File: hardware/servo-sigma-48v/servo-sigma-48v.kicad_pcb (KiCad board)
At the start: 4 copper layers, 74.5 x 75.2 mm, 203 parts, among them J1 CONN_01X02, J10 Conn_01x03, J11 Conn_01x03, J12 Conn_01x05, J2 CONN_02X05, J3 CONN_01X03, J4 Conn_01x03, J5 Conn_01x05, J6 629_105_150_921, J7 CONN_01X02, J8 Conn_01x03, J9 Conn_01x03, Q1 STL160NS3LLH7, Q2 STL160NS3LLH7, Q3 STL160NS3LLH7, Q4 STL160NS3LLH7, Q5 STL160NS3LLH7, Q6 STL160NS3LLH7, Q7 STL160NS3LLH7, Q8 STL160NS3LLH7, SW1 SW_DIP_x04, U1 ST1S14, U10 OPA4374, U11 L6398, U12 SN65HVD75DGKR, U2 TPS70950, U3 SN65HVD75DGKR, U4 L6398, U5 STM32F405VGTx, U6 L6398, U7 L6398, U8 TPS70933, U9 OPA4374, Y1 ABM3-8.000MHZ-D2Y-T

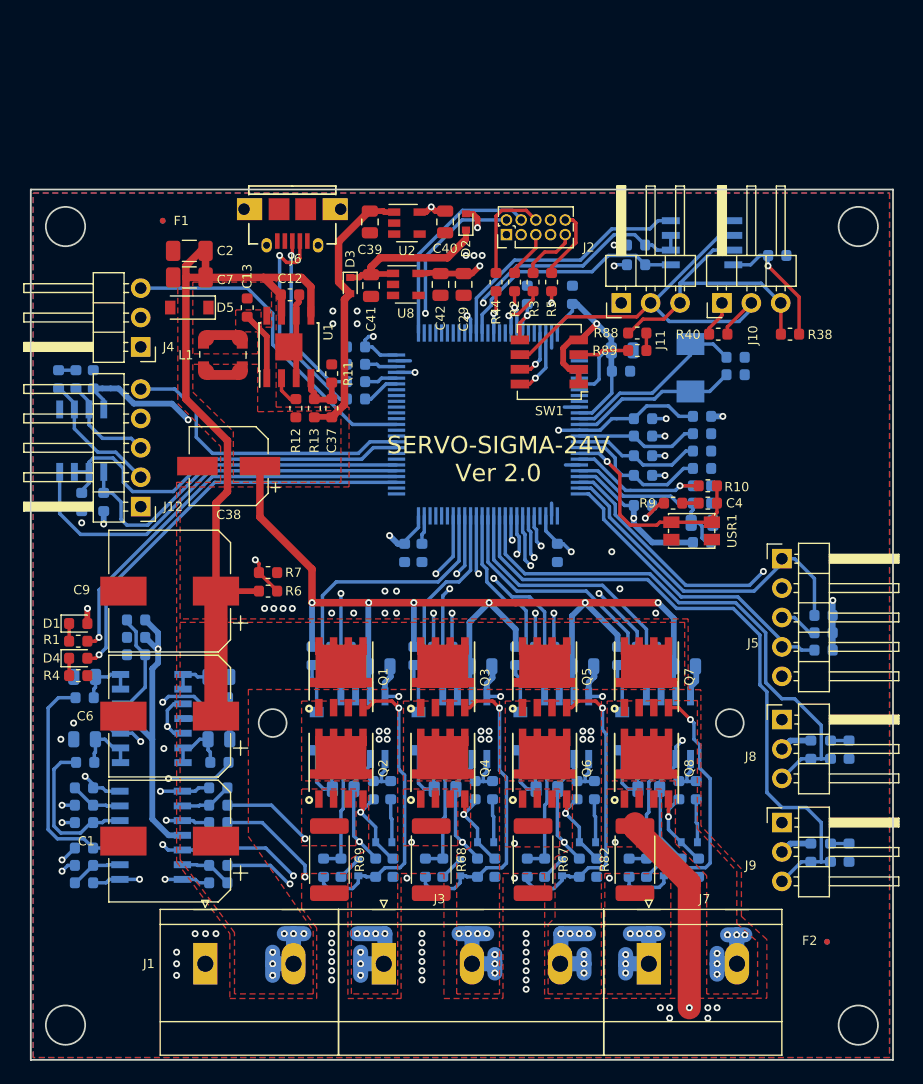
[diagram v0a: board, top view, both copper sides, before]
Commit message: completed routing
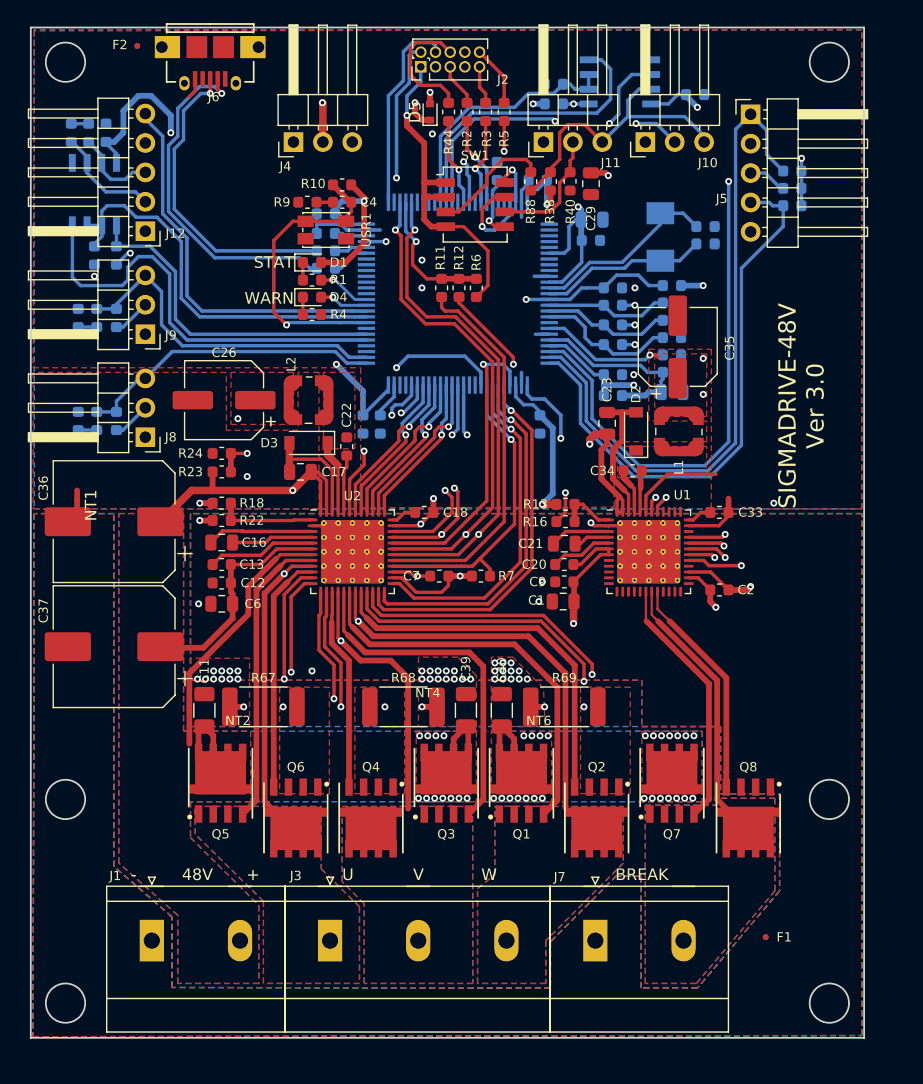
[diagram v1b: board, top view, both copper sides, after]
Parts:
- removed C38: 100uF, Capacitor_SMD:CP_Elec_6.3x7.7
- removed C41, C47, C50: 1uF 100V, Capacitor_SMD:C_0805_2012Metric
- removed C42, C44, C45, C46: 4.7uF 25V, Capacitor_SMD:C_0805_2012Metric
- removed C43: 100nF 50V, Capacitor_SMD:C_0603_1608Metric
- removed C48, C49: 100pF 100V, Capacitor_SMD:C_0603_1608Metric
- removed D10, D12, D13, D15, D16, D6, D7, D9: BAT30KFILM, Diodes_SMD:D_SOD-523
- removed D11, D14, D17, D8: STPS0560Z, Diodes_SMD:D_SOD-123
- removed R21, R27, R32, R37, R42, R56, R79, R80: 10k, Resistor_SMD:R_0603_1608Metric
- removed R25, R26, R29, R35, R36, R39, R54, R55, R74, R75, R78: 5, Resistor_SMD:R_0603_1608Metric
- removed R31, R41, R59, R60, R63, R64, R70, R71: 1.0k 0.1%, Resistor_SMD:R_0603_1608Metric
- removed R33, R34, R43, R53, R76, R77, R89: 21, Resistor_SMD:R_0603_1608Metric
- removed R57, R58, R61, R62, R65, R66, R72, R73: 10k 0.1%, Resistor_SMD:R_0603_1608Metric
- removed R82: 0.010 1%, Resistor_SMD:R_2512_6332Metric
- removed U10, U9: OPA4374, Package_SO:SOIC-14_3.9x8.7mm_P1.27mm
- removed U11, U4, U6, U7: L6398, Package_SO:SOIC-8_3.9x4.9mm_P1.27mm
- removed U8: TPS70933, Package_TO_SOT_SMD:SOT-23-5
- added L2: 22uH, Inductor_SMD:L_Wuerth_WE-TPC-3816, F.Cu at (100.5, 64.1)
- added NT1: Net-Tie_2, NetTie:NetTie-2_SMD_Pad0.5mm, F.Cu at (80.5, 73.2)
- added NT2: Net-Tie_2, NetTie:NetTie-2_SMD_Pad0.5mm, F.Cu at (94.4, 90.6)
- added NT4: Net-Tie_2, NetTie:NetTie-2_SMD_Pad0.5mm, F.Cu at (110.8, 90.6)
- added NT6: Net-Tie_2, NetTie:NetTie-2_SMD_Pad0.5mm, F.Cu at (120.4, 90.6)
- C1, C6: value 120uF -> 4.7uF 50V; footprint Capacitor_SMD:CP_Elec_10x10 -> Capacitor_SMD:C_0805_2012Metric
- C11: value 4.7uF 25V -> 1uF 100V; footprint Capacitor_SMD:C_0805_2012Metric -> Capacitor_SMD:C_1206_3216Metric; moved to F.Cu
- C12: value 100nF 100V -> 100nF
- C13: value 100nF 50V -> 1uF 16V
- C16, C21: value 100pF 100V -> 0.047uF 100V; footprint Capacitor_SMD:C_0603_1608Metric -> Capacitor_SMD:C_0805_2012Metric; moved to F.Cu
- C17: value 1uF 100V -> 4.7uF 50V; moved to F.Cu
- C18, C33: value 100pF 100V -> 1uF 16V; moved to F.Cu
- C2, C7: value 10uF 50V -> 100nF; footprint Capacitor_SMD:C_1206_3216Metric -> Capacitor_SMD:C_0603_1608Metric
- C20: value 1uF 100V -> 1uF 16V; footprint Capacitor_SMD:C_0805_2012Metric -> Capacitor_SMD:C_0603_1608Metric; moved to F.Cu
- C22, C34: value 1uF 100V -> 100nF; footprint Capacitor_SMD:C_0805_2012Metric -> Capacitor_SMD:C_0603_1608Metric; moved to F.Cu
- C23: value 100pF 100V -> 4.7uF 50V; footprint Capacitor_SMD:C_0603_1608Metric -> Capacitor_SMD:C_0805_2012Metric; moved to F.Cu
- C26: value 1uF 100V -> 100uF; footprint Capacitor_SMD:C_0805_2012Metric -> Capacitor_SMD:CP_Elec_6.3x7.7; moved to F.Cu
- C35: value 100pF 100V -> 100uF; footprint Capacitor_SMD:C_0603_1608Metric -> Capacitor_SMD:CP_Elec_6.3x7.7; moved to F.Cu
- C36: value 1uF 100V -> 120uF; footprint Capacitor_SMD:C_0805_2012Metric -> Capacitor_SMD:CP_Elec_10x10; moved to F.Cu
- C37: value 820pF/50V/10% -> 120uF; footprint Capacitor_SMD:C_0603_1608Metric -> Capacitor_SMD:CP_Elec_10x10
- C39: footprint Capacitor_SMD:C_0805_2012Metric -> Capacitor_SMD:C_1206_3216Metric
- C40: value 4.7uF 25V -> 1uF 100V; footprint Capacitor_SMD:C_0805_2012Metric -> Capacitor_SMD:C_1206_3216Metric
- C9: value 120uF -> 100nF; footprint Capacitor_SMD:CP_Elec_10x10 -> Capacitor_SMD:C_0603_1608Metric
- D2, D3: value BAT30KFILM -> STPS0560Z; footprint Diodes_SMD:D_SOD-523 -> Diode_SMD:D_SOD-123
- D5: value STPS0560Z -> BAT30KFILM; footprint Diodes_SMD:D_SOD-123 -> Diode_SMD:D_SOD-523
- L1: value 8.2uH -> 22uH
- R11: value 2.7k -> 21
- R12: value 47k -> 21
- R13: value 30k -> 28k
- R16: value 10k -> 8.45k; moved to F.Cu
- R18: value 5 -> 18k; moved to F.Cu
- R22: value 10k -> 3.3k; moved to F.Cu
- R23: value 21 -> 47k; moved to F.Cu
- R24: value 21 -> 4.7k; moved to F.Cu
- R6: value 47k -> 10k
- R7: value 4.7k -> 10k
- U1: value ST1S14 -> DRV8323RS; footprint Package_SO:SOIC-8-1EP_3.9x4.9mm_P1.27mm_EP2.35x2.35mm -> Package_DFN_QFN:QFN-48-1EP_7x7mm_P0.5mm_EP5.45x5.45mm_ThermalVias
- U2: value TPS70950 -> DRV8323RS; footprint Package_TO_SOT_SMD:SOT-23-5 -> Package_DFN_QFN:QFN-48-1EP_7x7mm_P0.5mm_EP5.45x5.45mm_ThermalVias
- moved F2 97.7 mm to (85.7, 33.5)
- moved F4 97.7 mm to (85.7, 33.5)
- moved R30 81.1 mm to (80.6, 57.0), turned to 90 degrees
- moved F1 80.9 mm to (140.0, 110.5)
- moved F3 80.9 mm to (140.0, 110.5)
- moved C52 78.4 mm to (82.2, 57.0), turned to 90 degrees
- moved R28 75.7 mm to (83.9, 57.0), turned to 90 degrees
- moved R20 72.4 mm to (80.6, 65.9), turned to 90 degrees
- moved C51 69.5 mm to (82.2, 65.9), turned to 90 degrees
- moved J9 69.3 mm to (86.4, 58.4), turned to 180 degrees
- moved R17 66.4 mm to (83.9, 65.9), turned to 90 degrees
- moved J8 60.2 mm to (86.4, 67.3), turned to 180 degrees
- moved C2 54.4 mm to (136.0, 80.5), turned to 0 degrees
- moved C39 43.0 mm to (114.1, 90.9)
- moved C40 42.5 mm to (117.2, 90.9)
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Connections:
- C1 pad 2: GND -> PGND
- C11 pad 1: GND -> VIN
- C11 pad 2: Net-(C11-Pad2) -> PGND
- C12 pad 2: GND -> PGND
- C13 pad 1: Net-(C13-Pad1) -> VIN
- C16 pad 1: GND -> Net-(C16-Pad1)
- C16 pad 2: /MCU/PWM_CL -> Net-(C16-Pad2)
- C17 pad 1: /MOSFETs/PHASE_C -> VIN
- C17 pad 2: Net-(C17-Pad2) -> GND
- C18 pad 1: GND -> Net-(C18-Pad1)
- C18 pad 2: /MCU/PWM_CH -> GND
- C2 pad 1: VIN -> +3V3
- C20 pad 1: GND -> VIN
- C20 pad 2: +15V -> Net-(C20-Pad2)
- C21 pad 1: GND -> Net-(C21-Pad1)
- C21 pad 2: /MCU/PWM_BL -> Net-(C21-Pad2)
- C22 pad 1: /MOSFETs/PHASE_B -> Net-(C22-Pad1)
- C23 pad 1: GND -> +5V
- C23 pad 2: /MCU/PWM_BH -> GND
- C26 pad 1: GND -> +5V
- C26 pad 2: +15V -> GND
- C33 pad 1: GND -> Net-(C33-Pad1)
- C33 pad 2: /MCU/PWM_AL -> GND
- C34 pad 1: /MOSFETs/PHASE_A -> Net-(C34-Pad1)
- C35 pad 1: GND -> +3V3
- C35 pad 2: /MCU/PWM_AH -> GND
- C36 pad 1: GND -> VIN
- C36 pad 2: +15V -> PGND
- C37 pad 1: +15V -> VIN
- C37 pad 2: Net-(C37-Pad2) -> PGND
- C39 pad 1: GND -> VIN
- C39 pad 2: +15V -> PGND
- C4 pad 2: /MCU/PC3 -> /MCU/PD11
- C40 pad 1: GND -> VIN
- C40 pad 2: +5V -> PGND
- C51 pad 2: /MCU/PB0 -> /MCU/PB12
- C52 pad 2: /MCU/PB1 -> /MCU/PB13
- C6 pad 2: GND -> PGND
- C7 pad 1: VIN -> +3V3
- C9 pad 2: GND -> PGND
- D2 pad 1: Net-(C41-Pad2) -> Net-(C34-Pad2)
- D2 pad 2: /MCU/EXT_5V -> GND
- D3 pad 1: Net-(C41-Pad2) -> Net-(C22-Pad2)
- D3 pad 2: +15V -> GND
- D5 pad 1: Net-(C13-Pad2) -> +5V
- D5 pad 2: GND -> /MCU/EXT_5V
- J1 pad 1: GND -> PGND
- J3 pad 1: /MOSFETs/PHASE_C -> /MOSFETs/PHASE_A
- J3 pad 3: /MOSFETs/PHASE_A -> /MOSFETs/PHASE_C
- J4 pad 3: /MCU/PWM -> /MCU/PB4
- J7 pad 1: /MOSFETs/R_ISENSE_P -> PGND
- J8 pad 3: /MCU/PB0 -> /MCU/PB12
- J9 pad 3: /MCU/PB1 -> /MCU/PB13
- L1 pad 1: Net-(C13-Pad2) -> Net-(C34-Pad2)
- L1 pad 2: +15V -> +3V3
- Q1 pad 2: Net-(D10-Pad2) -> /MOSFETs/GHC
- Q2 pad 2: Net-(D9-Pad2) -> /MOSFETs/GLC
- Q3 pad 2: Net-(D13-Pad2) -> /MOSFETs/GHB
- Q4 pad 2: Net-(D12-Pad2) -> /MOSFETs/GLB
- Q5 pad 2: Net-(D16-Pad2) -> /MOSFETs/GHA
- Q6 pad 2: Net-(D15-Pad2) -> /MOSFETs/GLA
- Q7 pad 2: Net-(D6-Pad2) -> /MOSFETs/GHR
- Q8 pad 1: GND -> PGND
- Q8 pad 2: Net-(D7-Pad2) -> /MOSFETs/GLR
- R10 pad 2: /MCU/PC3 -> /MCU/PD11
- R11 pad 1: GND -> /MCU/DRV_SDO
- R11 pad 2: Net-(C37-Pad2) -> Net-(R11-Pad2)
- R12 pad 1: Net-(R12-Pad1) -> /MCU/DRV_SDO
- R12 pad 2: +15V -> Net-(R12-Pad2)
- R13 pad 1: Net-(C37-Pad2) -> Net-(R13-Pad1)
- R13 pad 2: +15V -> +3V3
- R16 pad 1: Net-(R16-Pad1) -> GND
- R16 pad 2: +3V3 -> Net-(R13-Pad1)
- R17 pad 2: /MCU/PB0 -> /MCU/PB12
- R18 pad 1: +15V -> Net-(R18-Pad1)
- R18 pad 2: Net-(D8-Pad2) -> +5V
- R22 pad 1: Net-(D10-Pad2) -> GND
- R22 pad 2: /MOSFETs/PHASE_C -> Net-(R18-Pad1)
- R23 pad 1: /MOSFETs/GATE_CL -> VIN
- R23 pad 2: Net-(D9-Pad2) -> /MCU/VBAT_ADC
- R24 pad 1: /MOSFETs/GATE_CH -> /MCU/VBAT_ADC
- R24 pad 2: Net-(D10-Pad2) -> GND
- R28 pad 2: /MCU/PB1 -> /MCU/PB13
- R6 pad 1: VIN -> +3V3
- R6 pad 2: /MCU/VBAT_ADC -> /MCU/DRV_SDO
- R67 pad 2: GND -> PGND
- R68 pad 2: GND -> PGND
- R69 pad 2: GND -> PGND
- R7 pad 1: /MCU/VBAT_ADC -> +3V3
- R7 pad 2: GND -> /MCU/DRV_FAULT
- R88 pad 2: Net-(R88-Pad2) -> /MCU/B_TERM_R120
- U1 pad 1: Net-(C13-Pad1) -> Net-(R13-Pad1)
- U1 pad 2: Net-(R12-Pad1) -> PGND
- U1 pad 3: GND -> Net-(C21-Pad2)
- U1 pad 4: Net-(C37-Pad2) -> Net-(C21-Pad1)
- U1 pad 5: VIN -> Net-(C20-Pad2)
- U1 pad 6: GND -> VIN
- U1 pad 8: Net-(C13-Pad2) -> Net-(U1-Pad8)
- U1 pad 9: GND -> Net-(U1-Pad9)
- U2 pad 1: +15V -> Net-(R18-Pad1)
- U2 pad 2: GND -> PGND
- U2 pad 3: Net-(U2-Pad3) -> Net-(C16-Pad2)
- U2 pad 4: Net-(U2-Pad4) -> Net-(C16-Pad1)
- U2 pad 5: +5V -> Net-(C13-Pad2)
- U5 pad 26: /MCU/PA3 -> /MCU/DRV2_CS
- U5 pad 29: /MCU/PA4 -> /MCU/DRV1_CS
- U5 pad 30: /MCU/IA_FB -> /MOSFETs/DRV_SOC
- U5 pad 31: /MCU/IB_FB -> /MOSFETs/DRV_SOB
- U5 pad 32: /MCU/IC_FB -> /MOSFETs/DRV_SOA
- U5 pad 33: /MCU/IR_FB -> /MCU/DRV_FAULT
- U5 pad 45: /MCU/PE14 -> /MCU/GATE_ENABLE
- U5 pad 46: /MCU/PE15 -> /MCU/DRV_CAL
- U5 pad 53: /MCU/LED_WARN -> /MCU/PB14
- U5 pad 54: /MCU/LED_STATUS -> /MCU/PB15
- U5 pad 61: /MCU/PD14 -> /MCU/LED_WARN
- U5 pad 62: /MCU/PD15 -> /MCU/LED_STATUS
- U5 pad 63: /MCU/PWM -> /MCU/PC6
- U5 pad 78: /MCU/PC10 -> /MCU/DRV_CLK
- U5 pad 79: /MCU/PC11 -> /MCU/DRV_SDO
- U5 pad 80: /MCU/PC12 -> /MCU/DRV_SDI
- USR1 pad 2: /MCU/PC3 -> /MCU/PD11
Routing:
- net GND: track 216.8 -> 95.6 mm, vias 74 -> 15
- net +15V: track 119.4 -> 0.00 mm, vias 6 -> 0
- net /MCU/DRV_CLK: track 0.00 -> 71.5 mm, vias 0 -> 3
- net /MCU/DRV_SDI: track 0.00 -> 69.2 mm, vias 0 -> 3
- net /MCU/IB_FB: track 64.9 -> 0.00 mm, vias 2 -> 0
- net /MCU/IR_FB: track 62.8 -> 0.00 mm, vias 2 -> 0
- net /MOSFETs/R_ISENSE_P: track 60.3 -> 0.00 mm, vias 9 -> 0
- net /MCU/PB1: track 56.7 -> 0.00 mm
- net /MCU/GATE_ENABLE: track 0.00 -> 56.6 mm, vias 0 -> 4
- net /MCU/IC_FB: track 56.4 -> 0.00 mm, vias 2 -> 0
- net /MCU/IA_FB: track 56.0 -> 0.00 mm, vias 2 -> 0
- net VIN: track 74.7 -> 126.3 mm, vias 6 -> 38
- net /MCU/PB0: track 47.0 -> 0.00 mm
- net Net-(R12-Pad2): track 0.00 -> 42.0 mm, vias 0 -> 2
- net +5V: track 165.5 -> 203.6 mm, vias 1 -> 5
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- added copper zone on F.Cu, net +3V3
- added copper zone on F.Cu, net +5V
- added copper zone on B.Cu, net /MOSFETs/PHASE_A
- added copper zone on In2.Cu, net /MOSFETs/PHASE_A
- added copper zone on B.Cu, net /MOSFETs/PHASE_B
- added copper zone on In2.Cu, net /MOSFETs/PHASE_B
- added copper zone on B.Cu, net /MOSFETs/PHASE_C
- added copper zone on In2.Cu, net /MOSFETs/PHASE_C
- added copper zone on B.Cu, net /MOSFETs/PHASE_R
- added copper zone on In1.Cu, net /MOSFETs/PHASE_R
- added copper zone on In2.Cu, net /MOSFETs/PHASE_R
- added copper zone on In1.Cu, net GND
- added copper zone on In2.Cu, net GND
- added copper zone on F.Cu, net Net-(C22-Pad2)
- added copper zone on F.Cu, net Net-(C34-Pad2)
- added copper zone on B.Cu, net PGND
- added copper zone on F.Cu, net PGND
- added copper zone on In1.Cu, net PGND
- added copper zone on In2.Cu, net PGND
- added copper zone on B.Cu, net VIN
- added copper zone on In1.Cu, net VIN
- added copper zone on In2.Cu, net VIN
- removed copper zone on F.Cu, net +15V
- removed copper zone on F.Cu, net /MOSFETs/R_ISENSE_P
- removed copper zone on F.Cu, net Net-(C13-Pad2)
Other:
- board size 74.5 x 75.2 mm -> 72 x 87.3 mm
- board text added: "+"
- board text added: "-"
- board text added: "48V"
- board text added: "BREAK"
- board text added: "SIGMADRIVE-48V Ver 3.0"
- board text added: "STAT"
- board text added: "U"
- board text added: "V"
- board text added: "W"
- board text added: "WARN"
- board text removed: "SERVO-SIGMA-24V Ver 2.0"
